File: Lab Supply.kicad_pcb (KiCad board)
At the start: 2 copper layers, 134.9 x 116.8 mm, 88 parts, among them M1 Fan_4pin, Q1 TIP121, Q2 2N3904, Q3 TIP121, Q5 2N3904, SW1 ENABLE, U1 LM324, U2 LM7812_TO220, U3 MCP4922, U4 LM7805_TO220, U5 LM4040DBZ-2.0, U6 MCP3202

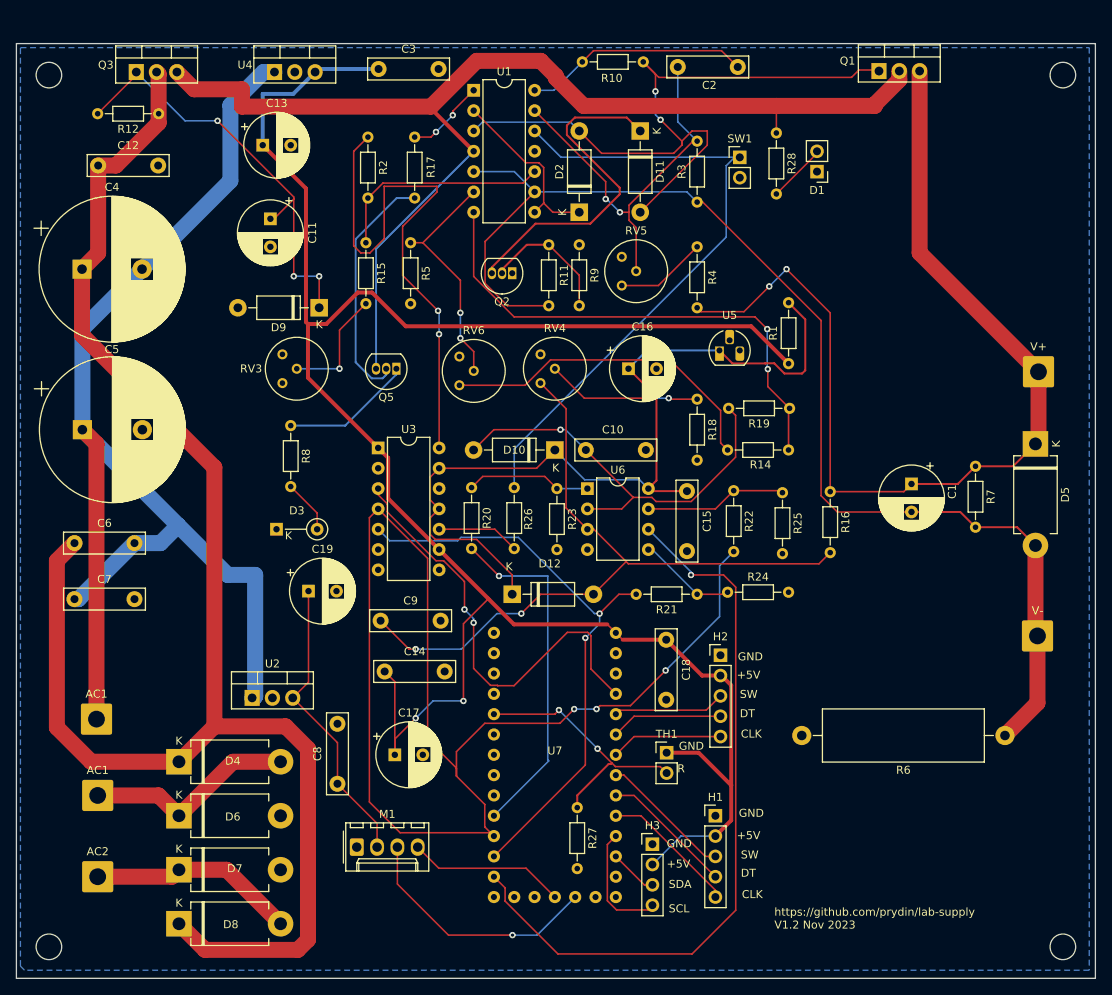
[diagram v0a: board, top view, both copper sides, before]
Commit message: WIP
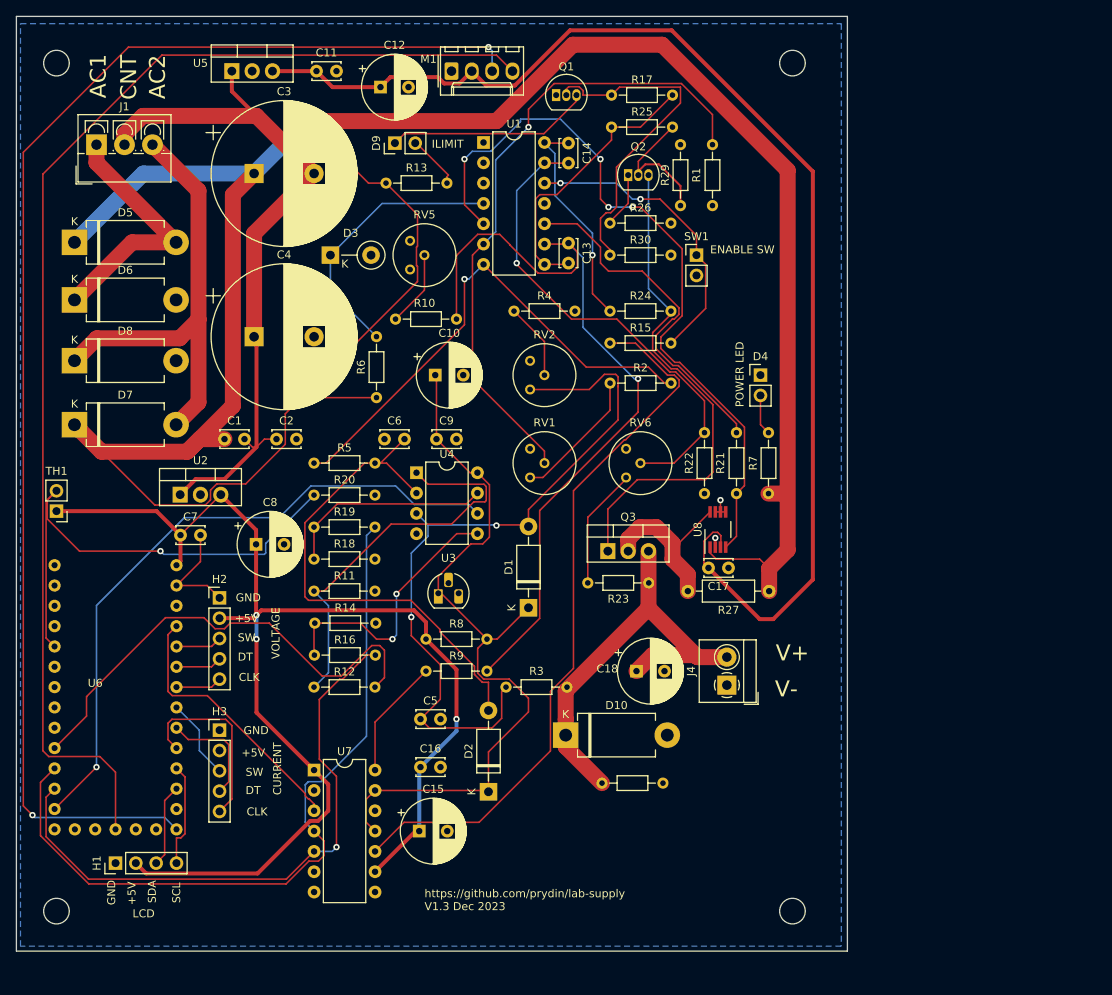
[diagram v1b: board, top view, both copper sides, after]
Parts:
- removed AC1 (x2): AC1, Connector_Wire:SolderWire-1.5sqmm_1x01_D1.7mm_OD3.9mm
- removed AC2: AC2, Connector_Wire:SolderWire-1.5sqmm_1x01_D1.7mm_OD3.9mm
- removed C19: 10u, Capacitor_THT:CP_Radial_D8.0mm_P3.50mm
- removed D11, D12: 1N4001, Diode_THT:D_DO-41_SOD81_P10.16mm_Horizontal
- removed Q5: 2N3904, Package_TO_SOT_THT:TO-92_Inline
- removed RV3: 22k, Potentiometer_THT:Potentiometer_Bourns_3339H_Vertical
- removed RV4: 10k, Potentiometer_THT:Potentiometer_Bourns_3339H_Vertical
- removed V+: V+, Connector_Wire:SolderWire-1.5sqmm_1x01_D1.7mm_OD3.9mm
- removed V-: V-, Connector_Wire:SolderWire-1.5sqmm_1x01_D1.7mm_OD3.9mm
- added J1: INPUT, TerminalBlock_4Ucon:TerminalBlock_4Ucon_1x03_P3.50mm_Vertical, F.Cu at (57.0, 48.2)
- added J4: OUTPUT, TerminalBlock_4Ucon:TerminalBlock_4Ucon_1x02_P3.50mm_Horizontal, F.Cu at (135.8, 115.8)
- added R13: 1.5k, Resistor_THT:R_Axial_DIN0204_L3.6mm_D1.6mm_P7.62mm_Horizontal, F.Cu at (93.2, 53.0)
- added R29: 1k, Resistor_THT:R_Axial_DIN0204_L3.6mm_D1.6mm_P7.62mm_Horizontal, F.Cu at (130.0, 55.8)
- added R30: 1k, Resistor_THT:R_Axial_DIN0204_L3.6mm_D1.6mm_P7.62mm_Horizontal, F.Cu at (121.2, 62.0)
- added RV1: 20k, Potentiometer_THT:Potentiometer_Bourns_3339H_Vertical, F.Cu at (111.2, 89.8)
- added RV2: 10k, Potentiometer_THT:Potentiometer_Bourns_3339H_Vertical, F.Cu at (111.2, 78.8)
- added U8: INA225, Package_SO:VSSOP-8_3.0x3.0mm_P0.65mm, F.Cu at (134.7, 96.3)
- C1, C11: value 100u -> 100n; footprint Capacitor_THT:CP_Radial_D8.0mm_P3.50mm -> Capacitor_THT:C_Disc_D3.4mm_W2.1mm_P2.50mm
- C10, C12, C15, C8: value 100n -> 10u; footprint Capacitor_THT:C_Rect_L10.0mm_W2.5mm_P7.50mm_MKS4 -> Capacitor_THT:CP_Radial_D8.0mm_P3.50mm
- C13: value 10u -> 1n; footprint Capacitor_THT:CP_Radial_D8.0mm_P3.50mm -> Capacitor_THT:C_Disc_D3.4mm_W2.1mm_P2.50mm
- C14: value 100n -> 1n; footprint Capacitor_THT:C_Rect_L10.0mm_W2.5mm_P7.50mm_MKS4 -> Capacitor_THT:C_Disc_D3.4mm_W2.1mm_P2.50mm
- C16, C17: value 10u -> 100n; footprint Capacitor_THT:CP_Radial_D8.0mm_P3.50mm -> Capacitor_THT:C_Disc_D3.4mm_W2.1mm_P2.50mm
- C18: value 100n -> 100u; footprint Capacitor_THT:C_Rect_L10.0mm_W2.5mm_P7.50mm_MKS4 -> Capacitor_THT:CP_Radial_D8.0mm_P3.50mm
- C2: value 10nf -> 100n; footprint Capacitor_THT:C_Rect_L10.0mm_W2.5mm_P7.50mm_MKS4 -> Capacitor_THT:C_Disc_D3.4mm_W2.1mm_P2.50mm
- C3: value 100n -> 4700u; footprint Capacitor_THT:C_Rect_L10.0mm_W2.5mm_P7.50mm_MKS4 -> Capacitor_THT:CP_Radial_D18.0mm_P7.50mm
- C5: value 4700u -> 100n; footprint Capacitor_THT:CP_Radial_D18.0mm_P7.50mm -> Capacitor_THT:C_Disc_D3.4mm_W2.1mm_P2.50mm
- C6, C7, C9: footprint Capacitor_THT:C_Rect_L10.0mm_W2.5mm_P7.50mm_MKS4 -> Capacitor_THT:C_Disc_D3.4mm_W2.1mm_P2.50mm
- D1: value POWER -> 1N4001; footprint Connector_PinHeader_2.54mm:PinHeader_1x02_P2.54mm_Vertical -> Diode_THT:D_DO-41_SOD81_P10.16mm_Horizontal
- D10: value 1N4001 -> 1N5400; footprint Diode_THT:D_DO-41_SOD81_P10.16mm_Horizontal -> Diode_THT:D_DO-201AD_P12.70mm_Horizontal
- D3: value I_LIMIT_ON -> 1N4752A; footprint Diode_THT:D_DO-35_SOD27_P5.08mm_Vertical_KathodeUp -> Diode_THT:D_DO-41_SOD81_P5.08mm_Vertical_KathodeUp
- D4: value 1N5400 -> POWER; footprint Diode_THT:D_DO-201AD_P12.70mm_Horizontal -> Connector_PinHeader_2.54mm:PinHeader_1x02_P2.54mm_Vertical
- D9: value 1N4751ATR -> I_LIMIT_ON; footprint Diode_THT:D_DO-41_SOD81_P10.16mm_Horizontal -> Connector_PinHeader_2.54mm:PinHeader_1x02_P2.54mm_Vertical
- H1: value Current -> Display; footprint Connector_PinHeader_2.54mm:PinHeader_1x05_P2.54mm_Vertical -> Connector_PinHeader_2.54mm:PinHeader_1x04_P2.54mm_Vertical
- H3: value Display -> Current; footprint Connector_PinHeader_2.54mm:PinHeader_1x04_P2.54mm_Vertical -> Connector_PinHeader_2.54mm:PinHeader_1x05_P2.54mm_Vertical
- Q1: value TIP121 -> 2N3904; footprint Package_TO_SOT_THT:TO-220-3_Vertical -> Package_TO_SOT_THT:TO-92_Inline
- R1: value 1k -> 10k
- R10: value 10k -> 6.8k
- R11, R18: value 10k -> 470
- R12, R19: value 10k -> 100
- R14: value 22k -> 470
- R15: value 10k -> 47k
- R16: value 100k -> 100
- R2: value 47k -> 22k
- R20: value 100 -> 10k
- R21: value 100 -> 4.7k
- R22: value 100 -> 8.2k
- R23: value 470 -> 47k
- R24: value 470 -> 3k
- R25: value 470 -> 10k
- R26: value 47k -> 220
- R27: value 10k -> 0.05; footprint Resistor_THT:R_Axial_DIN0204_L3.6mm_D1.6mm_P7.62mm_Horizontal -> Resistor_THT:R_Axial_DIN0207_L6.3mm_D2.5mm_P10.16mm_Horizontal
- R28: value 1.5k -> 8.2k
- R3: value 10k -> 100k
- R4: value 47k -> 10k
- R6: value 0.5 -> 100; footprint Resistor_THT:R_Axial_Power_L20.0mm_W6.4mm_P25.40mm -> Resistor_THT:R_Axial_DIN0204_L3.6mm_D1.6mm_P7.62mm_Horizontal
- R7: value 8.2k -> 1.5k
- R8: value 1.5k -> 1k
- R9: value 22k -> 10k
- RV5, RV6: value 20k -> 10k
- U2: value LM7812_TO220 -> LM7805_TO220
- U3: value MCP4922 -> LM4040DBZ-2.0; footprint Package_DIP:DIP-14_W7.62mm -> Package_TO_SOT_THT:TO-92_HandSolder
- U4: value LM7805_TO220 -> MCP3202; footprint Package_TO_SOT_THT:TO-220-3_Vertical -> Package_DIP:DIP-8_W7.62mm
- U5: value LM4040DBZ-2.0 -> LM7812_TO220; footprint Package_TO_SOT_THT:TO-92_HandSolder -> Package_TO_SOT_THT:TO-220-3_Vertical
- U6: value MCP3202 -> ~; footprint Package_DIP:DIP-8_W7.62mm -> Arduino:Itsy Bitsy 5V
- U7: value ~ -> MCP4922; footprint Arduino:Itsy Bitsy 5V -> Package_DIP:DIP-14_W7.62mm
- moved D5 122.7 mm to (54.2, 60.4), turned to 0 degrees
- moved M1 97.7 mm to (101.4, 39.0)
- moved R6 89.2 mm to (92.0, 79.8), turned to 90 degrees
- moved D4 87.3 mm to (140.0, 77.0)
- moved C1 86.1 mm to (73.0, 85.0), turned to 0 degrees
- moved R28 84.1 mm to (120.2, 128.0), turned to 0 degrees
- moved Q3 84.0 mm to (120.9, 99.0)
- moved TH1 82.0 mm to (52.0, 94.0), turned to 180 degrees
- moved H1 75.2 mm to (59.4, 138.0), turned to 90 degrees
- moved R12 74.3 mm to (84.2, 116.0), turned to 0 degrees
- moved D2 73.3 mm to (106.0, 129.1)
- moved D8 71.6 mm to (54.2, 75.2)
- moved U5 70.2 mm to (73.9, 39.0)
- moved C14 69.9 mm to (116.0, 48.0), turned to -90 degrees
- moved C2 68.4 mm to (79.5, 85.0)
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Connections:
- C1 pad 1: V+ -> +36V
- C1 pad 2: ISENSE -> +15V
- C10 pad 1: GND -> VREF
- C10 pad 2: Net-(D10-A) -> V-
- C11 pad 1: Net-(D9-K) -> +12V
- C11 pad 2: GND -> V-
- C12 pad 1: +36V -> +12V
- C12 pad 2: GND -> V-
- C13 pad 1: +5V -> Net-(U1C--)
- C13 pad 2: GND -> Net-(C13-Pad2)
- C14 pad 1: +5V -> Net-(C14-Pad1)
- C14 pad 2: GND -> Net-(U1D--)
- C15 pad 1: VREF -> +5V
- C15 pad 2: GND -> V-
- C16 pad 1: VREF -> +5V
- C16 pad 2: GND -> V-
- C17 pad 1: +5V -> V-
- C17 pad 2: GND -> +12V
- C18 pad 1: +5V -> V+
- C18 pad 2: GND -> V-
- C2 pad 1: Net-(U1D--) -> +15V
- C2 pad 2: Net-(C2-Pad2) -> V-
- C3 pad 1: +5V -> +36V
- C3 pad 2: GND -> +15V
- C4 pad 1: +36V -> +15V
- C4 pad 2: CENTER -> V-
- C5 pad 1: CENTER -> Net-(D1-A)
- C5 pad 2: GND -> V-
- C6 pad 1: +36V -> V-
- C6 pad 2: CENTER -> Net-(D2-A)
- C7 pad 1: CENTER -> +5V
- C7 pad 2: GND -> V-
- C8 pad 1: Net-(M1-+) -> +5V
- C8 pad 2: GND -> V-
- C9 pad 1: Net-(D12-A) -> VREF
- C9 pad 2: GND -> V-
- D1 pad 1: GND -> VREF
- D10 pad 1: VREF -> V+
- D10 pad 2: Net-(D10-A) -> V-
- D2 pad 1: Net-(D2-K) -> VREF
- D2 pad 2: Net-(D11-A) -> Net-(D2-A)
- D3 pad 1: GND -> +28V
- D3 pad 2: Net-(D3-A) -> V-
- D4 pad 1: +36V -> V-
- D4 pad 2: AC1 -> Net-(D4-A)
- D5 pad 1: V+ -> +36V
- D5 pad 2: ISENSE -> AC1
- D6 pad 2: GND -> V-
- D7 pad 1: AC2 -> +36V
- D7 pad 2: GND -> AC2
- D8 pad 1: +36V -> AC2
- D8 pad 2: AC2 -> V-
- D9 pad 2: GND -> Net-(D9-A)
- H1 pad 1: GND -> V-
- H1 pad 3: Net-(H1-SW) -> Net-(H1-SDA)
- H1 pad 4: Net-(H1-DT) -> Net-(H1-SCL)
- H2 pad 1: GND -> V-
- H3 pad 1: GND -> V-
- H3 pad 3: Net-(H3-SDA) -> Net-(H3-SW)
- H3 pad 4: Net-(H3-SCL) -> Net-(H3-DT)
- M1 pad 1: GND -> V-
- M1 pad 2: Net-(M1-+) -> +12V
- Q1 pad 1: Net-(D11-A) -> V-
- Q1 pad 2: +28V -> Net-(Q1-B)
- Q1 pad 3: V+ -> Net-(D9-K)
- Q2 pad 1: GND -> Net-(Q2-E)
- Q2 pad 3: Net-(D11-K) -> Net-(Q2-C)
- Q3 pad 1: Net-(D9-K) -> Net-(Q2-C)
- Q3 pad 2: +36V -> Net-(Q3-C)
- Q3 pad 3: +28V -> V+
- R1 pad 1: +5V -> Net-(U1B--)
- R1 pad 2: VREF -> V-
- R10 pad 1: Net-(C2-Pad2) -> Net-(U1C--)
- R10 pad 2: Net-(D11-A) -> Net-(R10-Pad2)
- R11 pad 1: Net-(Q2-B) -> Net-(U4-~{CS}/SHDN)
- R11 pad 2: ISENSE -> V-
- R12 pad 1: +36V -> Net-(U4-~{CS}/SHDN)
- R12 pad 2: Net-(D9-K) -> Net-(U6-A5)
- R14 pad 1: Net-(R14-Pad1) -> Net-(U4-DIN)
- R14 pad 2: Net-(R14-Pad2) -> V-
- R15 pad 1: Net-(U1C-+) -> V_VSET
- R15 pad 2: Net-(R15-Pad2) -> Net-(SW1-A)
- R16 pad 1: V+ -> Net-(U4-DIN)
- R16 pad 2: Net-(D12-A) -> Net-(U6-MOSI)
- R17 pad 1: Net-(Q5-B) -> Net-(Q1-B)
- R17 pad 2: Net-(R17-Pad2) -> Net-(C13-Pad2)
- R18 pad 1: Net-(R18-Pad1) -> Net-(U4-CLK)
- R18 pad 2: GND -> V-
- R19 pad 1: Net-(R14-Pad2) -> Net-(U4-CLK)
- R19 pad 2: Net-(D10-A) -> Net-(U6-SCK)
- R2 pad 1: V_ISET -> Net-(R2-Pad1)
- R2 pad 2: Net-(U1C-+) -> Net-(R2-Pad2)
- R20 pad 1: Net-(U6-~{CS}/SHDN) -> Net-(U6-A0)
- R20 pad 2: Net-(U7-A5) -> V-
- R21 pad 1: Net-(U6-DIN) -> Net-(U1C-+)
- R21 pad 2: Net-(U3-SDI) -> ISENSE
- R22 pad 1: Net-(U6-CLK) -> V-
- R22 pad 2: Net-(U3-SCK) -> Net-(U1D--)
- R23 pad 1: Net-(U6-~{CS}/SHDN) -> Net-(R23-Pad1)
- R23 pad 2: GND -> V+
- R24 pad 1: Net-(U6-DIN) -> Net-(C14-Pad1)
- R24 pad 2: GND -> Net-(Q2-C)
- R25 pad 1: Net-(U6-CLK) -> Net-(C13-Pad2)
- R25 pad 2: GND -> Net-(Q2-B)
- R26 pad 1: V_VSET -> Net-(Q2-E)
- R26 pad 2: Net-(SW1-A) -> V-
- R27 pad 1: Net-(U7-A0) -> +36V
- R27 pad 2: GND -> Net-(Q3-C)
- R28 pad 1: +28V -> V+
- R28 pad 2: Net-(D1-A) -> V-
- R3 pad 1: ISENSE -> V+
- R3 pad 2: Net-(U1D--) -> Net-(D1-A)
- R4 pad 2: V+ -> V-
- R5 pad 1: Net-(U1B--) -> Net-(R2-Pad2)
- R5 pad 2: GND -> Net-(D2-A)
- R6 pad 1: ISENSE -> +36V
- R6 pad 2: GND -> +28V
- R7 pad 1: V+ -> +36V
- R7 pad 2: ISENSE -> Net-(D4-A)
- R8 pad 1: Net-(Q5-E) -> +5V
- R8 pad 2: Net-(D3-A) -> VREF
- R9 pad 1: GND -> V_ISET
- R9 pad 2: Net-(Q2-B) -> Net-(U1C--)
- RV5 pad 1: Net-(R4-Pad1) -> unconnected-(RV5-Pad1)
- RV5 pad 2: Net-(U1D--) -> Net-(R10-Pad2)
- RV5 pad 3: unconnected-(RV5-Pad3) -> V-
- RV6 pad 1: Net-(R14-Pad1) -> Net-(R23-Pad1)
- RV6 pad 2: Net-(U1B--) -> Net-(U1D--)
- SW1 pad 2: GND -> V-
- TH1 pad 2: Net-(U7-A0) -> Net-(U6-A0)
- U1 pad 1: Net-(R17-Pad2) -> (no net)
- U1 pad 11: GND -> V-
- U1 pad 14: Net-(C2-Pad2) -> Net-(C14-Pad1)
- U1 pad 2: Net-(D2-K) -> (no net)
- U1 pad 3: Net-(D11-A) -> (no net)
- U1 pad 7: Net-(R14-Pad2) -> Net-(R2-Pad2)
- U1 pad 8: Net-(D2-K) -> Net-(C13-Pad2)
- U1 pad 9: ISENSE -> Net-(U1C--)
- U2 pad 1: CENTER -> +15V
- U2 pad 2: GND -> V-
- U2 pad 3: Net-(M1-+) -> +5V
- U3 pad 1: +5V -> VREF
- U3 pad 2: unconnected-(U3-NC-Pad2) -> V-
- U3 pad 3: Net-(U3-~{CS}) -> (no net)
- U4 pad 1: CENTER -> Net-(U4-~{CS}/SHDN)
- U4 pad 2: GND -> Net-(D2-A)
- U4 pad 3: +5V -> Net-(D1-A)
- U5 pad 1: VREF -> +15V
- U5 pad 2: GND -> V-
- U5 pad 3: (no net) -> +12V
- U6 pad 1: Net-(U6-~{CS}/SHDN) -> unconnected-(U6-RST-Pad1)
- U6 pad 2: Net-(D10-A) -> unconnected-(U6-5V-Pad2)
- U6 pad 3: Net-(D12-A) -> unconnected-(U6-AREF-Pad3)
- U6 pad 4: GND -> V-
- U6 pad 5: Net-(U6-DIN) -> Net-(U6-A0)
- U6 pad 6: Net-(U6-DOUT) -> unconnected-(U6-A1-Pad6)
- U6 pad 7: Net-(U6-CLK) -> unconnected-(U6-A2-Pad7)
- U6 pad 8: VREF -> unconnected-(U6-A3-Pad8)
- U7 pad 1: unconnected-(U7-RST-Pad1) -> +5V
- U7 pad 10: Net-(U7-A5) -> V_VSET
- U7 pad 11: Net-(U3-SCK) -> VREF
- U7 pad 12: Net-(U3-SDI) -> V-
- U7 pad 13: Net-(U6-DOUT) -> VREF
- U7 pad 14: unconnected-(U7-3.3V-Pad14) -> V_ISET
- U7 pad 3: unconnected-(U7-AREF-Pad3) -> Net-(U6-D13)
- U7 pad 4: GND -> Net-(U6-SCK)
- U7 pad 5: Net-(U7-A0) -> Net-(U6-MOSI)
- U7 pad 8: unconnected-(U7-A3-Pad8) -> V-
- U7 pad 9: unconnected-(U7-A4-Pad9) -> +5V
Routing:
- net +12V: track 0.00 -> 157.3 mm
- net CENTER: track 153.9 -> 0.00 mm
- net Net-(U3-SCK): track 153.1 -> 0.00 mm, vias 3 -> 0
- net Net-(M1-Tacho): track 31.5 -> 168.8 mm, vias 1 -> 2
- net Net-(M1-PWM): track 19.7 -> 155.1 mm
- net +36V: track 196.0 -> 325.8 mm, vias 0 -> 1
- net +28V: track 144.6 -> 34.4 mm
- net +5V: track 267.1 -> 164.8 mm, vias 2 -> 3
- net Net-(U1C--): track 0.00 -> 98.2 mm, vias 0 -> 1
- net Net-(U6-SCK): track 0.00 -> 95.1 mm
- net Net-(U6-DOUT): track 92.0 -> 0.00 mm, vias 1 -> 0
- net Net-(D12-A): track 90.1 -> 0.00 mm, vias 2 -> 0
- net +15V: track 0.00 -> 90.1 mm
- net Net-(D11-A): track 89.4 -> 0.00 mm, vias 2 -> 0
- net Net-(D1-A): track 7.44 -> 92.9 mm, vias 0 -> 2
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- added copper zone on B.Cu, net V-
- removed copper zone on B.Cu, net GND
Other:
- board size 134.9 x 116.8 mm -> 103.9 x 116.8 mm
- board text added: "AC1"
- board text added: "AC2"
- board text added: "CNT"
- board text added: "CURRENT"
- board text added: "ENABLE SW"
- board text added: "ILIMIT"
- board text added: "LCD"
- board text added: "POWER LED"
- board text added: "V+"
- board text added: "V-"
- board text added: "VOLTAGE"
- board text added: "https://github.com/prydin/lab-supply V1.3 Dec 2023"
- board text removed: "R"
- board text removed: "https://github.com/prydin/lab-supply V1.2 Nov 2023"
